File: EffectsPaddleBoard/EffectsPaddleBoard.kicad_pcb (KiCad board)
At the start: 4 copper layers, 113.6 x 84.6 mm, 121 parts, among them J1 Conn_01x03_Pin, J2 Conn_01x06_Pin, J3 Barrel_Jack, J4 Conn_01x04_Pin, J5 AudioJack2, J6 AudioJack2, SW1 SW_SPDT, SW2 SW_Push, SW3 SW_SPDT, U1 STM32F405RGTx, U2 TPS54233, U3 TLV320AIC3100, U4 TPS54233, U5 MCP6401T-xLT, U6 MCP6401T-xLT, U7 MCP6401T-xLT, Y1 16MHz

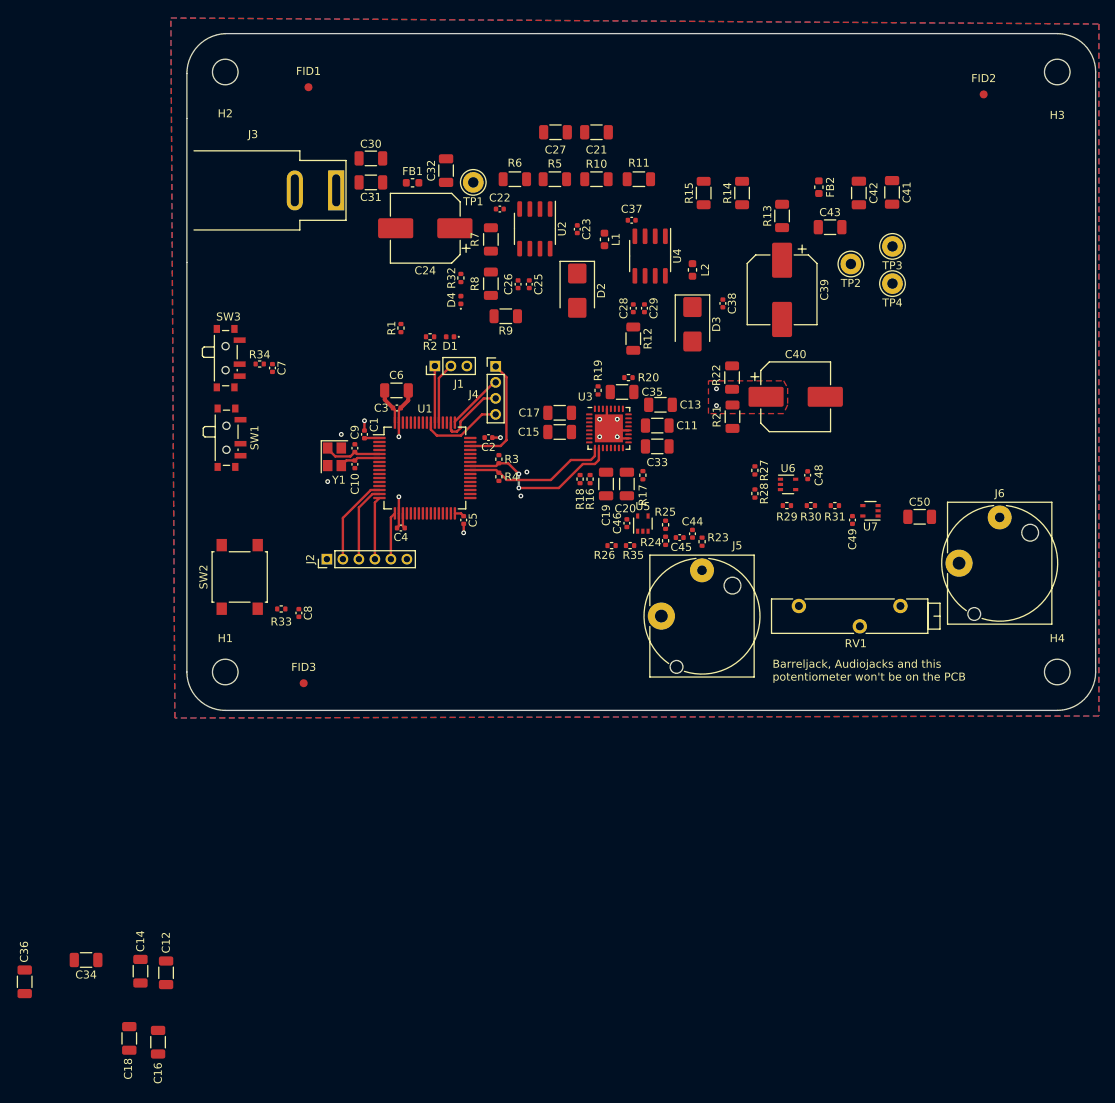
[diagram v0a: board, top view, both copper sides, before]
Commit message: Corrected the board, now all parts should be right
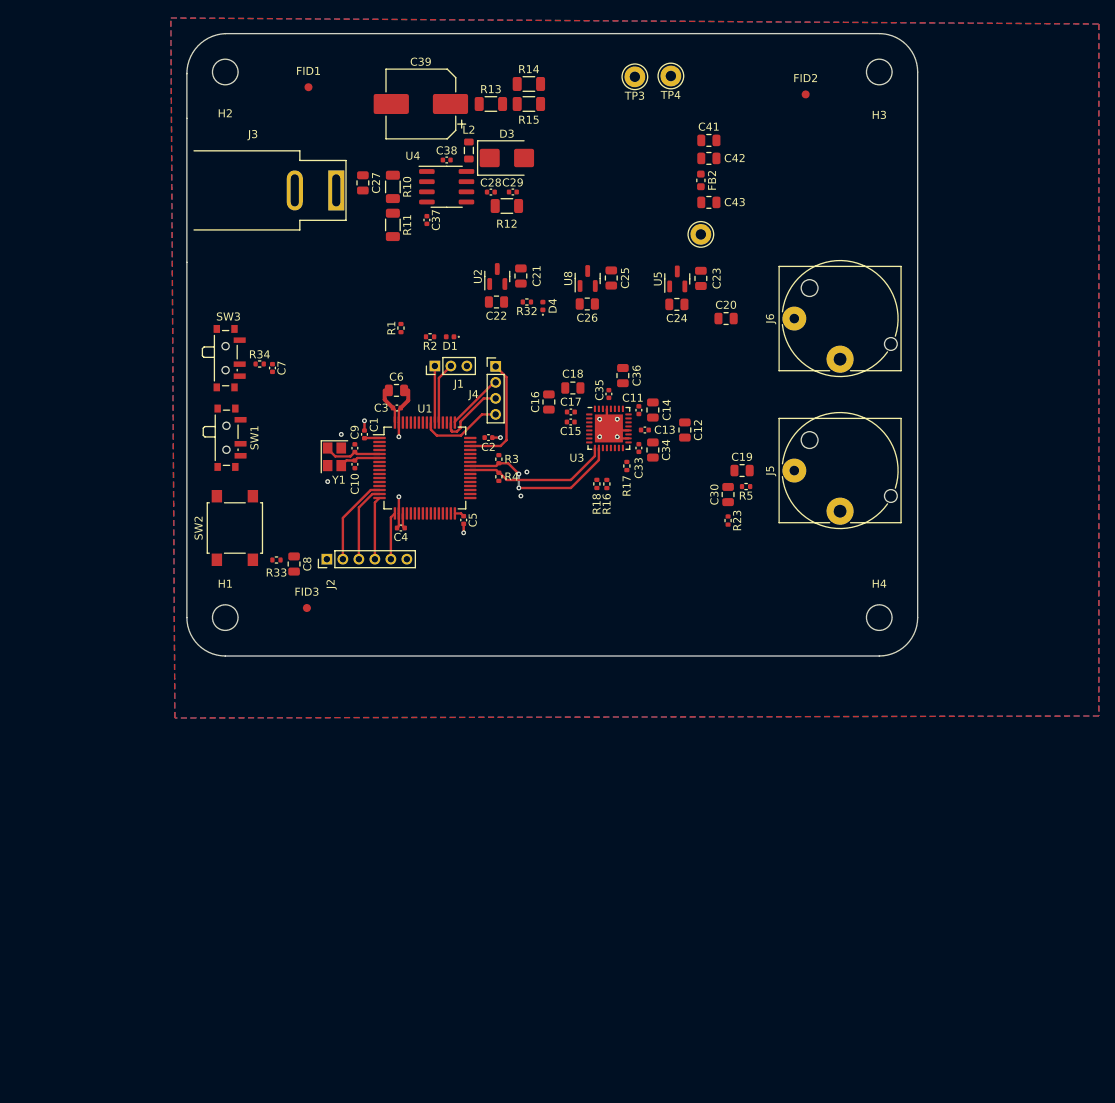
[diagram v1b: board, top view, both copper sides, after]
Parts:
- removed C31, C32: 1u, Capacitor_SMD:C_1206_3216Metric
- removed C40: 470u, Capacitor_SMD:CP_Elec_8x10.5
- removed C44: 220p, Capacitor_SMD:C_0402_1005Metric
- removed C45: 10n, Capacitor_SMD:C_0402_1005Metric
- removed C46, C48, C49: 100n, Capacitor_SMD:C_0402_1005Metric
- removed C50: 10u, Capacitor_SMD:C_1206_3216Metric
- removed D2: B230, Diode_SMD:D_SMB
- removed FB1: 600, Inductor_SMD:L_0603_1608Metric
- removed L1: 15u, Inductor_SMD:L_0603_1608Metric
- removed R19, R20, R24, R25, R26, R31: 10k, Resistor_SMD:R_0402_1005Metric
- removed R21: 4k7, Resistor_SMD:R_1206_3216Metric
- removed R22: 3k9, Resistor_SMD:R_1206_3216Metric
- removed R27, R30: 3k9, Resistor_SMD:R_0402_1005Metric
- removed R28, R29: 4k7, Resistor_SMD:R_0402_1005Metric
- removed R35: 0, Resistor_SMD:R_0402_1005Metric
- removed R6: 68.1k, Resistor_SMD:R_1206_3216Metric
- removed R7: 10.2k, Resistor_SMD:R_1206_3216Metric
- removed R8: 3.24k, Resistor_SMD:R_1206_3216Metric
- removed R9: 30.9k, Resistor_SMD:R_1206_3216Metric
- removed RV1: 100k, Potentiometer_THT:Potentiometer_Bourns_3005_Horizontal
- removed TP1: TestPoint, Connector_Pin:Pin_D1.3mm_L11.0mm
- removed U6, U7: MCP6401T-xLT, Package_TO_SOT_SMD:SOT-353_SC-70-5
- added U8: TPS7A0518PDBZ, Package_TO_SOT_SMD:SOT-23, F.Cu at (171.1, 76.8)
- C11, C13, C15, C17, C33, C35: value 100u -> 100n; footprint Capacitor_SMD:C_1206_3216Metric -> Capacitor_SMD:C_0402_1005Metric
- C12, C14: value 22m -> 22u; footprint Capacitor_SMD:C_1206_3216Metric -> Capacitor_SMD:C_0805_2012Metric
- C16, C18, C34, C36: value 10m -> 10u; footprint Capacitor_SMD:C_1206_3216Metric -> Capacitor_SMD:C_0805_2012Metric
- C19: value 1m -> 1u; footprint Capacitor_SMD:C_1206_3216Metric -> Capacitor_SMD:C_0805_2012Metric
- C20: value 1m -> 47u; footprint Capacitor_SMD:C_1206_3216Metric -> Capacitor_SMD:C_0805_2012Metric
- C21, C30: value 10u -> 1u; footprint Capacitor_SMD:C_1206_3216Metric -> Capacitor_SMD:C_0805_2012Metric
- C22: value 15n -> 1u; footprint Capacitor_SMD:C_0402_1005Metric -> Capacitor_SMD:C_0805_2012Metric
- C23, C8: value 100n -> 1u; footprint Capacitor_SMD:C_0402_1005Metric -> Capacitor_SMD:C_0805_2012Metric
- C24: value 470u -> 1u; footprint Capacitor_SMD:CP_Elec_8x10.5 -> Capacitor_SMD:C_0805_2012Metric
- C25, C26: value 220p -> 1u; footprint Capacitor_SMD:C_0402_1005Metric -> Capacitor_SMD:C_0805_2012Metric
- C27, C41, C42, C43, C6: footprint Capacitor_SMD:C_1206_3216Metric -> Capacitor_SMD:C_0805_2012Metric
- FB2: value 600 -> 100
- L2: footprint Inductor_SMD:L_0603_1608Metric -> Inductor_SMD:L_0805_2012Metric
- R33: value 10k -> 220
- R5: value 332k -> 0; footprint Resistor_SMD:R_1206_3216Metric -> Resistor_SMD:R_0402_1005Metric
- U2: value TPS54233 -> TPS7A0533PDBZ; footprint Package_SO:SOIC-8_3.9x4.9mm_P1.27mm -> Package_TO_SOT_SMD:SOT-23
- U5: value MCP6401T-xLT -> TPS7A0533PDBZ; footprint Package_TO_SOT_SMD:SOT-353_SC-70-5 -> Package_TO_SOT_SMD:SOT-23
- moved C36 106.5 mm to (175.5, 89.0)
- moved C18 98.4 mm to (169.2, 90.5), turned to 180 degrees
- moved C34 95.3 mm to (179.2, 98.2), turned to -90 degrees
- moved C14 95.0 mm to (179.2, 93.2)
- moved C12 93.9 mm to (183.2, 95.8), turned to -90 degrees
- moved C16 93.8 mm to (166.2, 92.2), turned to 90 degrees
- moved C30 61.3 mm to (188.7, 103.8), turned to 90 degrees
- moved C39 50.8 mm to (150.2, 55.0), turned to 180 degrees
- moved R5 45.2 mm to (190.9, 102.8), turned to 180 degrees
- moved R13 39.0 mm to (159.0, 55.0), turned to 0 degrees
- moved C38 38.9 mm to (153.5, 62.0), turned to 0 degrees
- moved TP3 38.6 mm to (177.0, 51.6)
- moved TP4 38.0 mm to (181.5, 51.5)
- moved J6 35.7 mm to (196.9, 81.8), turned to 90 degrees
- moved C24 32.9 mm to (182.2, 80.0), turned to 0 degrees
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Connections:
- C19 pad 2: Analog_In1 -> Net-(C19-Pad2)
- C20 pad 1: /Codec/Analog_In_R -> /Codec/HPL
- C20 pad 2: Analog_In2 -> /Codec/AudioOutBoard
- C21 pad 1: /Barreljack_in -> GND
- C21 pad 2: GND -> +5V
- C22 pad 1: /SS3v3 -> GND
- C22 pad 2: GND -> +3.3V
- C23 pad 1: /b3v3 -> GND
- C23 pad 2: /ph3v3out -> +5V
- C24 pad 1: +3.3V -> GND
- C24 pad 2: GND -> +3.3VA
- C25 pad 1: /comp3v3 -> GND
- C25 pad 2: GND -> +5V
- C26 pad 1: /comp3v3 -> GND
- C26 pad 2: Net-(C26-Pad2) -> +1V8
- C30 pad 1: +3.3VA -> /Codec/Analog_In_R
- C30 pad 2: GND -> Net-(C30-Pad2)
- J5 pad T: /Analog_FrontBackend/AudioInBoard -> Net-(C19-Pad2)
- J6 pad T: /Analog_FrontBackend/AudioOutBoard -> /Codec/AudioOutBoard
- R23 pad 1: /Analog_FrontBackend/AudioInBoard -> /Codec/Analog_In_R
- R23 pad 2: /Analog_FrontBackend/InLP -> GND
- R5 pad 1: /Barreljack_in -> Net-(C19-Pad2)
- R5 pad 2: /en3v3 -> Net-(C30-Pad2)
- U2 pad 1: /b3v3 -> GND
- U2 pad 2: /Barreljack_in -> +3.3V
- U2 pad 3: /en3v3 -> +5V
- U3 pad 19: Audio_M -> unconnected-(U3-SPKM-Pad19)
- U3 pad 22: Audio_P -> unconnected-(U3-SPKP-Pad22)
- U3 pad 23: Audio_M -> unconnected-(U3-SPKM-Pad19)
- U3 pad 26: Audio_P -> unconnected-(U3-SPKP-Pad22)
- U3 pad 30: /Codec/HPR -> unconnected-(U3-HPR-Pad30)
- U5 pad 1: Analog_In1 -> GND
- U5 pad 2: GND -> +3.3VA
- U5 pad 3: /Analog_FrontBackend/InSigAudio -> +5V
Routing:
- net +1V8: vias 2 -> 0
- removed copper zone on F.Cu, net +1V8
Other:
- board size 113.6 x 84.6 mm -> 91.3 x 77.8 mm
- board text removed: "Barreljack, Audiojacks and this potentiometer won't be on the PCB"
- board text removed: "Would move them as close as possible to the codec"

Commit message: Layout completed
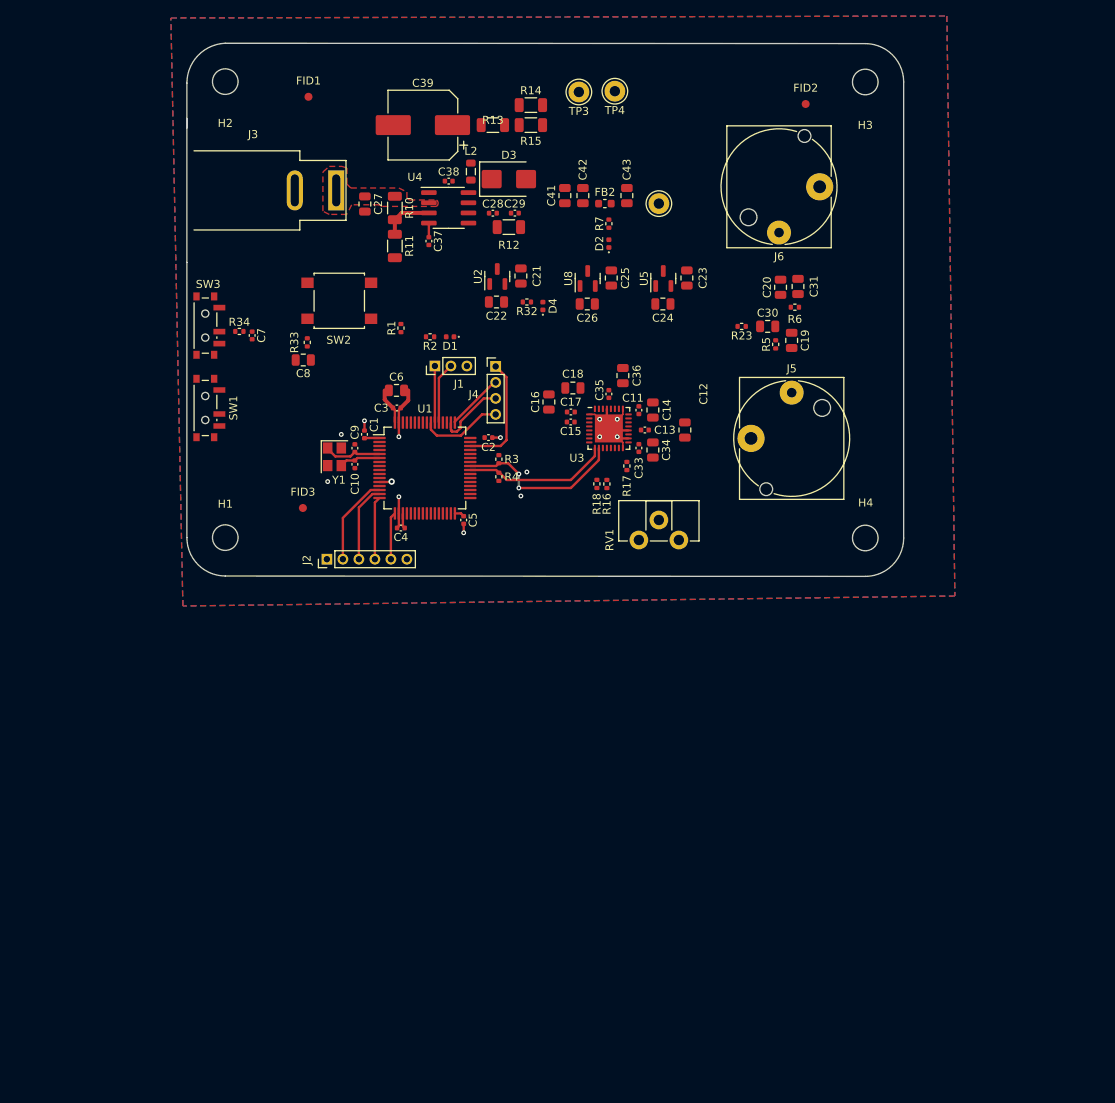
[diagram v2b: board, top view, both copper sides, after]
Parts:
- added C31: 47u, Capacitor_SMD:C_0805_2012Metric, F.Cu at (197.4, 77.8)
- added D2: LED, LED_SMD:LED_0402_1005Metric, F.Cu at (173.8, 72.5)
- added R6: 0, Resistor_SMD:R_0402_1005Metric, F.Cu at (197.0, 80.4)
- added R7: 220, Resistor_SMD:R_0402_1005Metric, F.Cu at (173.8, 70.0)
- added RV1: 10k, Potentiometer_THT:Potentiometer_ACP_CA9-H2,5_Horizontal, F.Cu at (177.5, 109.5)
- moved SW2 31.3 mm to (140.1, 79.6), turned to 0 degrees
- moved R33 27.5 mm to (136.1, 84.8), turned to -90 degrees
- moved C8 25.5 mm to (135.6, 87.0), turned to 180 degrees
- moved R23 24.3 mm to (190.3, 82.8), turned to 180 degrees
- moved C30 21.6 mm to (193.6, 82.8), turned to 0 degrees
- moved C41 19.3 mm to (168.2, 66.5), turned to 90 degrees
- moved R5 18.2 mm to (194.6, 85.0), turned to 90 degrees
- moved C19 17.4 mm to (196.6, 84.5), turned to -90 degrees
- moved C42 16.4 mm to (170.5, 66.5), turned to 90 degrees
- moved FID3 12.5 mm to (135.5, 105.5)
- moved FB2 12.3 mm to (173.2, 67.5), turned to 0 degrees
- moved J6 10.9 mm to (195.0, 71.1), turned to 180 degrees
- moved C43 10.3 mm to (176.0, 66.5), turned to 90 degrees
- moved H4 10.1 mm to (205.8, 109.2)
- moved H1 10.0 mm to (125.8, 109.2)
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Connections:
- R18 pad 1: /Codec/Volume -> +3.3VA
- R18 pad 2: GND -> /Codec/VolumeVDiv
- U3 pad 30: unconnected-(U3-HPR-Pad30) -> Net-(U3-HPR)
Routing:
- net GND: track 21.7 -> 32.8 mm, vias 13 -> 14
- net /en5v: track 0.00 -> 6.43 mm
- net /SS5v: track 0.00 -> 1.77 mm
- added copper zone on F.Cu, net /Barreljack_in
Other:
- board size 91.3 x 77.8 mm -> 89.6 x 66.6 mm
- board text removed: "In general, make yourself clear if you want the periapherals connected from the sides or from top."
- board text removed: "Make clear seperatrion between analog and digital parts of your circuit. E.g. now the ferrit pi filter is located on the opposit side of where it is needed."
- board text removed: "Mark clearly which connector does what. You don't want to grill your guitar."
- board text removed: "Move the switches to the pcb edge or change them to horizontal ones."
